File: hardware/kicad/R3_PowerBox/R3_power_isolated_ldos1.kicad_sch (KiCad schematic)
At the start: 12 parts, among them U4 ADM7150ACPZ-3.3-R7, U5 TPS7A2033PDBVR

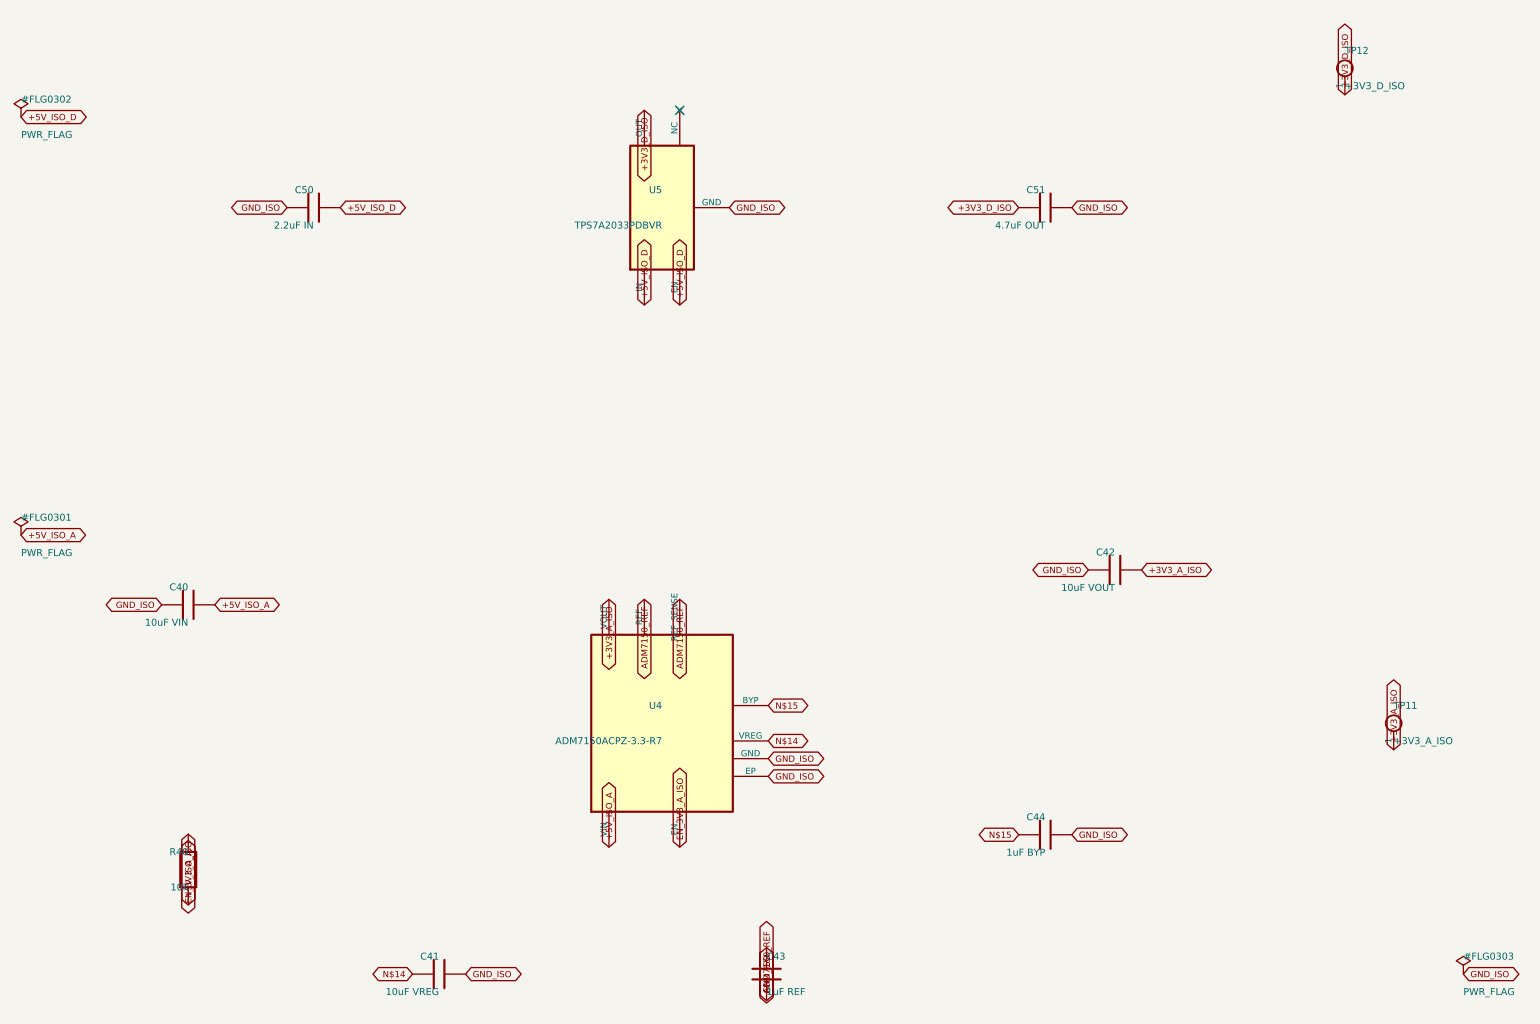
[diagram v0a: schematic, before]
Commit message: Finalize R3 PowerBox pre-placement corrections
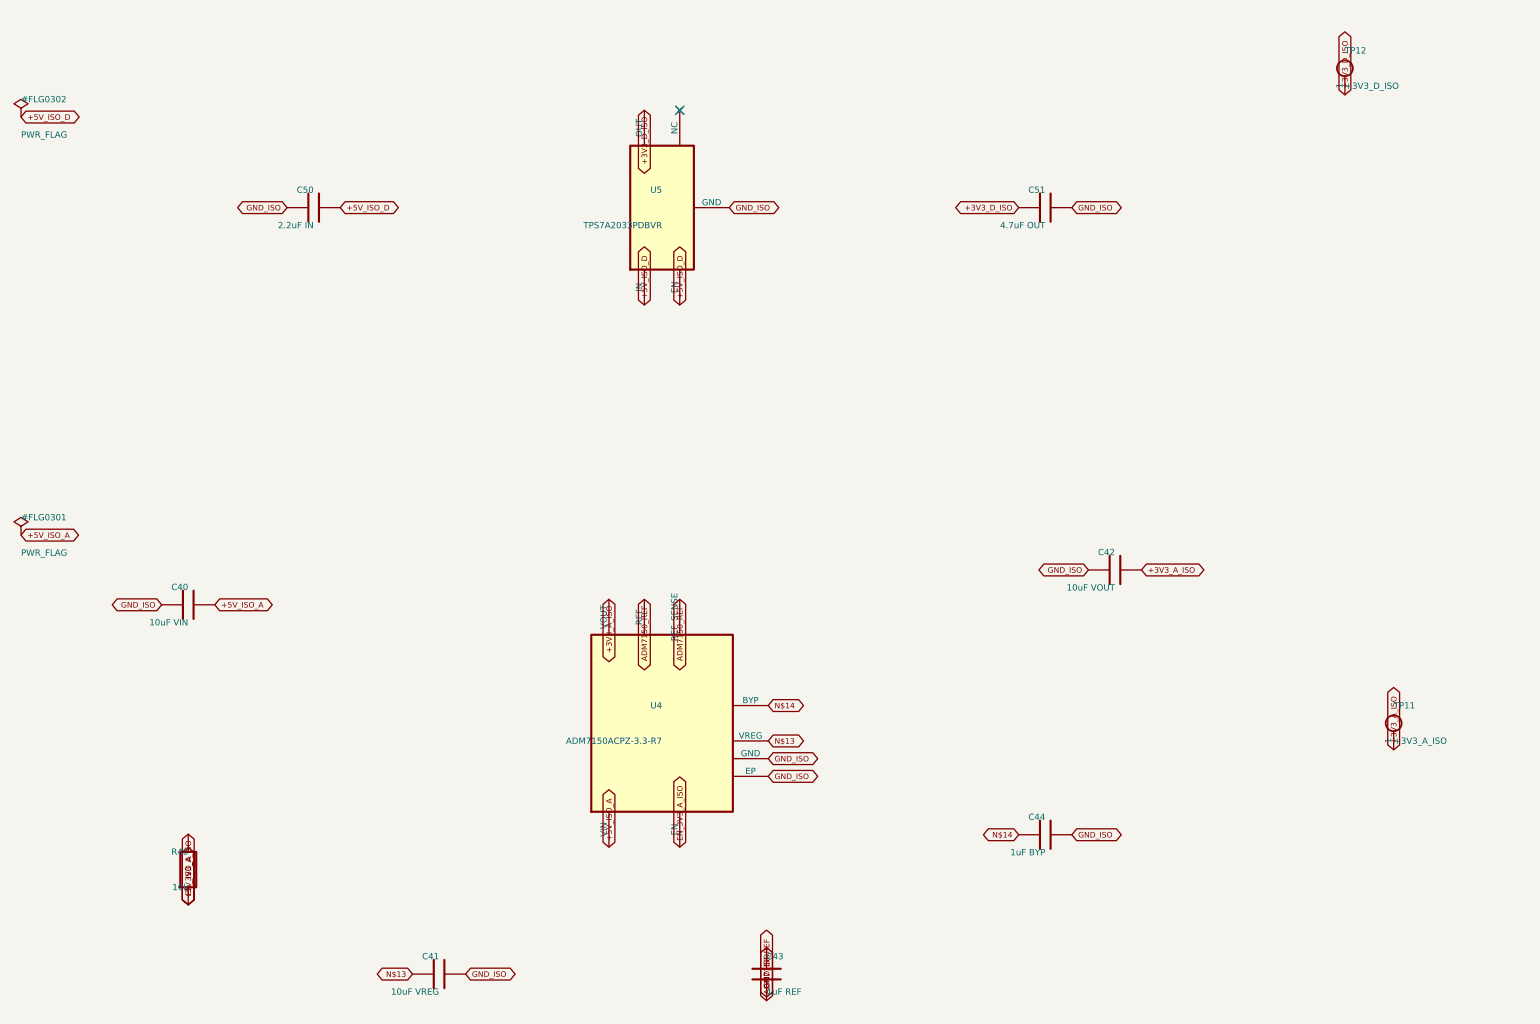
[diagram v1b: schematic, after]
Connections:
- net N$15 is gone; now on net N$14: C44.1, U4.3 (BYP)
- net N$14: no longer C41.1, U4.1 (VREG)
- new net N$13: C41.1, U4.1 (VREG)
